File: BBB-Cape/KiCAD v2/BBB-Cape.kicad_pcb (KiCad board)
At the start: 2 copper layers, 54.6 x 86.4 mm, 85 parts, among them J1 MOUNTING_HOLE, J10 Conn_01x02, J11 RJ45-TRANSFO, J12 DB9_Female, J2 MOUNTING_HOLE, J3 MOUNTING_HOLE, J4 MOUNTING_HOLE, J5 MOUNTING_HOLE, J6 MOUNTING_HOLE, J7 MOUNTING_HOLE, J8 MOUNTING_HOLE, J9 01x06_Stackable Header, P1 02x23_Stackable Header, P2 02x23_Stackable Header, SW1 W5500_RST, SW2 SYS_RST, SW3 Power, U1 LM25576MH, U2 WIZnet W5500, U3 MAX13433EETD, Y1 25MHz

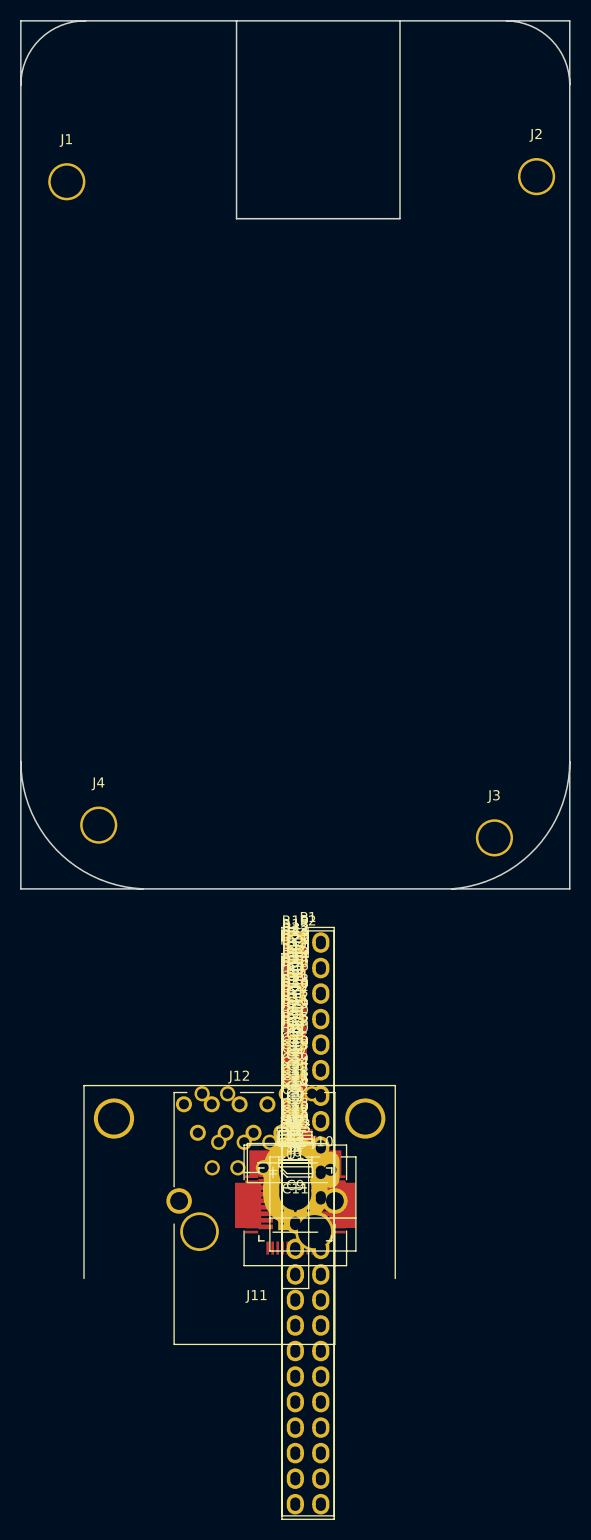
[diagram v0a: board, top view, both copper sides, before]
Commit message: Layout start for Rev3
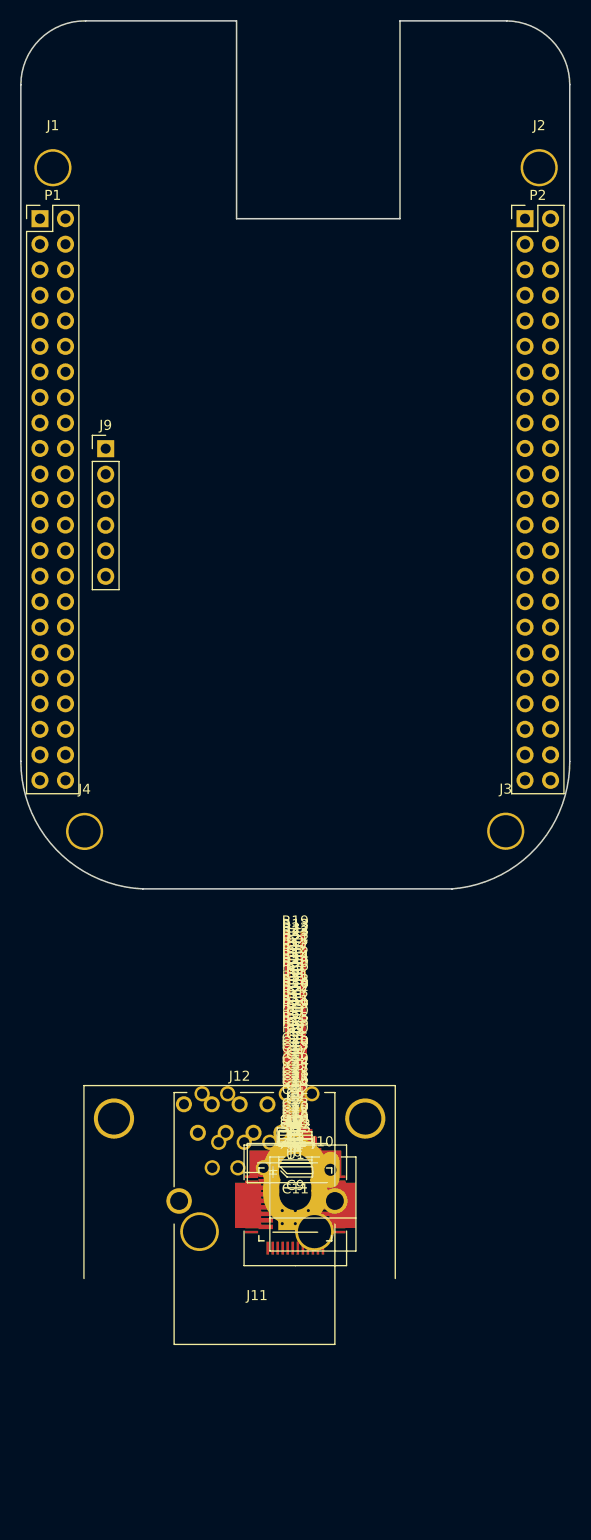
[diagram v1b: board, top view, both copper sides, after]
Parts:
- moved P1 76.2 mm to (112.6, 67.2)
- moved P2 75.7 mm to (160.8, 67.2)
- moved J9 72.0 mm to (119.1, 90.1)
- moved J1 1.96 mm to (113.9, 62.1)
- moved J4 1.54 mm to (117.0, 128.2)
- moved J3 1.30 mm to (158.9, 128.2)
- moved J2 0.92 mm to (162.2, 62.1)
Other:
- outline, holes or cut-outs redrawn
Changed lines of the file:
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@@
     (area 110.592799 47.458559 165.352801 198.739687)
     (thickness 1.6)
-    (drawings 11)
+    (drawings 12)
     (tracks 0)
     (zones 0)
@@
   )
   (module Mounting_Holes:MountingHole_3.2mm_M3_Pad (layer F.Cu)
-    (at 115.2398 63.5381)
+    (at 113.8578 62.1461)
     (descr "Mounting Hole 3.2mm, M3")
     (tags "mounting hole 3.2mm m3")
@@
   )
   (module Mounting_Holes:MountingHole_3.2mm_M3_Pad (layer F.Cu)
-    (at 161.9758 63.0301)
+    (at 162.2378 62.1461)
     (descr "Mounting Hole 3.2mm, M3")
     (tags "mounting hole 3.2mm m3")
@@
   )
   (module Mounting_Holes:MountingHole_3.2mm_M3_Pad (layer F.Cu)
-    (at 157.7848 128.8161)
+    (at 158.9078 128.1561)
     (descr "Mounting Hole 3.2mm, M3")
     (tags "mounting hole 3.2mm m3")
@@
   )
   (module Mounting_Holes:MountingHole_3.2mm_M3_Pad (layer F.Cu)
-    (at 118.4148 127.5461)
+    (at 117.0078 128.1761)
     (descr "Mounting Hole 3.2mm, M3")
     (tags "mounting hole 3.2mm m3")
@@
   )
   (module Pin_Headers:Pin_Header_Straight_1x06_Pitch2.54mm (layer F.Cu)
-    (at 137.9728 159.619499)
+    (at 119.1078 90.0961)
     (descr "Through hole straight pin header, 1x06, 2.54mm pitch, single row")
     (tags "Through hole pin header THT 1x06 2.54mm single row")
@@
   )
   (module Pin_Headers:Pin_Header_Straight_2x23_Pitch2.54mm (layer F.Cu)
-    (at 137.9728 139.05789)
+    (at 112.5678 67.2161)
     (descr "Through hole straight pin header, 2x23, 2.54mm pitch, double rows")
     (tags "Through hole pin header THT 2x23 2.54mm double row")
@@
   )
   (module Pin_Headers:Pin_Header_Straight_2x23_Pitch2.54mm (layer F.Cu)
-    (at 137.9728 139.400687)
+    (at 160.8278 67.2161)
     (descr "Through hole straight pin header, 2x23, 2.54mm pitch, double rows")
     (tags "Through hole pin header THT 2x23 2.54mm double row")
@@
     )
   )
+  (gr_line (start 122.8178 133.8961) (end 153.5678 133.8961) (layer Edge.Cuts) (width 0.15))
+  (gr_line (start 110.6678 53.8961) (end 110.6678 121.2061) (layer Edge.Cuts) (width 0.15))
+  (gr_line (start 132.1278 47.5361) (end 117.1078 47.5361) (layer Edge.Cuts) (width 0.15))
+  (gr_line (start 148.3878 47.5361) (end 159.0078 47.5361) (layer Edge.Cuts) (width 0.15))
+  (gr_line (start 165.2778 121.2061) (end 165.2778 53.8861) (layer Edge.Cuts) (width 0.15))
   (gr_line (start 148.3878 67.2161) (end 148.3878 47.5361) (layer Edge.Cuts) (width 0.15))
   (gr_line (start 132.1278 67.2161) (end 148.3838 67.2161) (layer Edge.Cuts) (width 0.15))
@@
   (gr_arc (start 123.3678 121.20626) (end 110.6678 121.20626) (angle -87.47303961) (layer Edge.Cuts) (width 0.15))
   (gr_arc (start 152.56764 121.22404) (end 165.2778 121.2215) (angle 85.5529637) (layer Edge.Cuts) (width 0.15))
-  (gr_line (start 165.2778 133.89356) (end 165.2778 47.53356) (layer Edge.Cuts) (width 0.15))
-  (gr_line (start 110.6678 133.89356) (end 165.2778 133.89356) (layer Edge.Cuts) (width 0.15))
-  (gr_line (start 110.6678 47.53356) (end 165.2778 47.53356) (layer Edge.Cuts) (width 0.15))
-  (gr_line (start 110.6678 133.89356) (end 110.6678 47.53356) (layer Edge.Cuts) (width 0.15))
 )
